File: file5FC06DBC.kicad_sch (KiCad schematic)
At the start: 29 parts, among them J7 SMA, U3 Si4463, U4 AS179-92LF, X1 TCXO 26 MHz

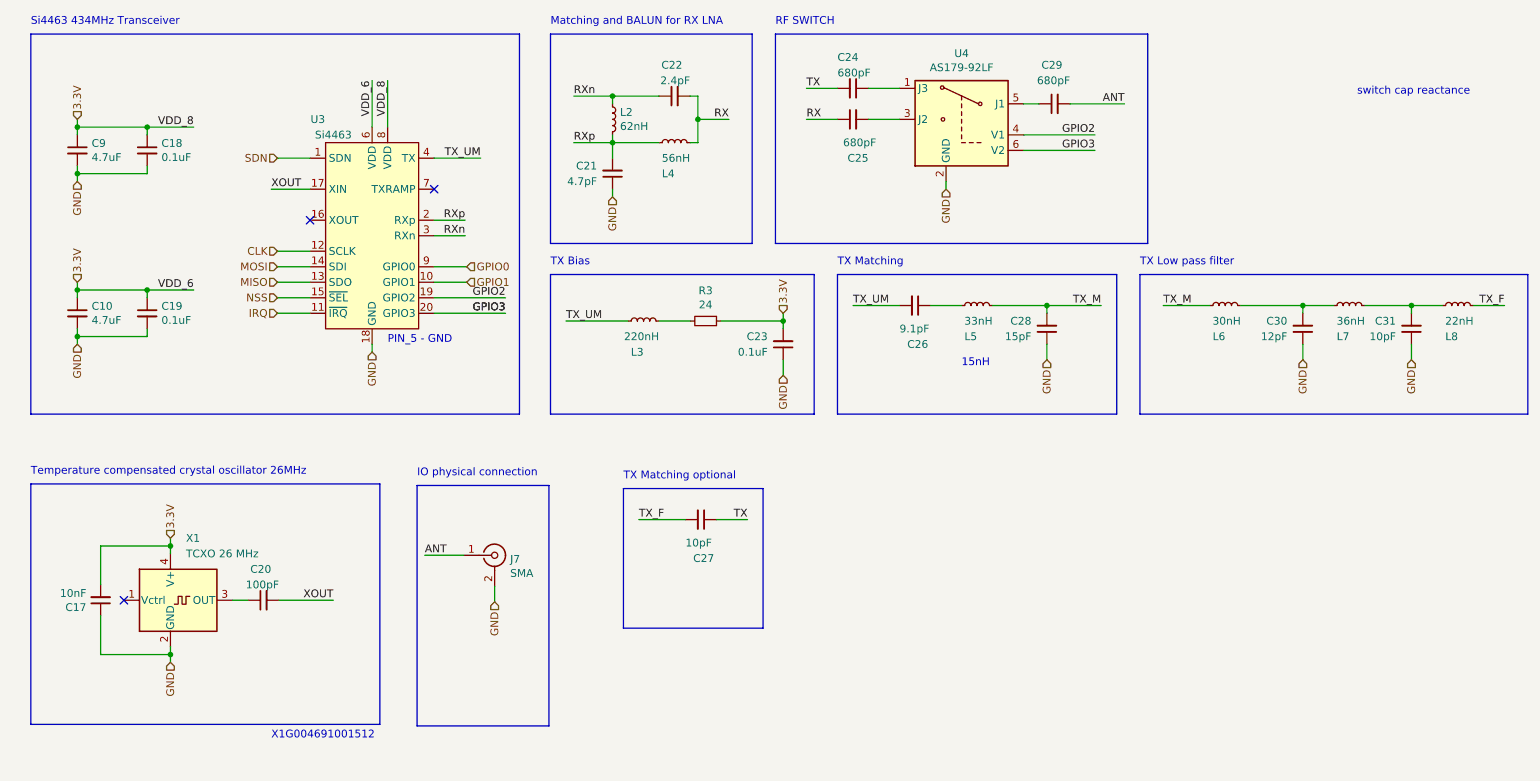
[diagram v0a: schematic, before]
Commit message: KiCad 0.2v
Schematics done.
Have to assign footprints to corresponding components.
Completely rework PCB.
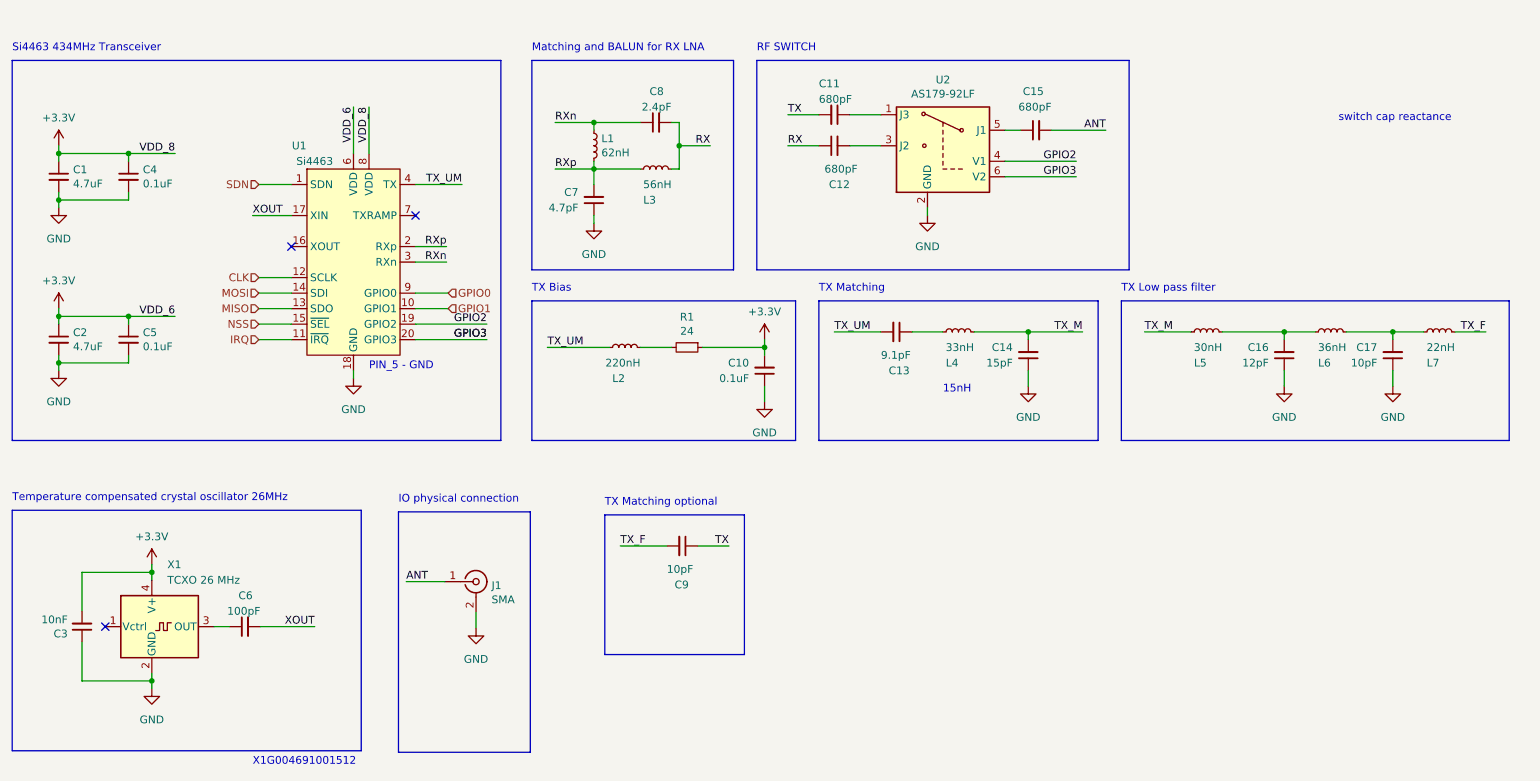
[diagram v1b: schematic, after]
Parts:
- removed C18, C19, C23: 0.1uF, Capacitor_SMD:C_0402_1005Metric, symbol Device:C_Small
- removed C20: 100pF, Capacitor_SMD:C_0402_1005Metric, symbol Device:C_Small
- removed C21: 4.7pF, Capacitor_SMD:C_0402_1005Metric, symbol Device:C_Small
- removed C22: 2.4pF, Capacitor_SMD:C_0402_1005Metric, symbol Device:C_Small
- removed C24, C25, C29: 680pF, Capacitor_SMD:C_0402_1005Metric, symbol Device:C_Small
- removed C26: 9.1pF, Capacitor_SMD:C_0402_1005Metric, symbol Device:C_Small
- removed C27, C31: 10pF, Capacitor_SMD:C_0402_1005Metric, symbol Device:C_Small
- removed C28: 15pF, Capacitor_SMD:C_0402_1005Metric, symbol Device:C_Small
- removed C30: 12pF, Capacitor_SMD:C_0402_1005Metric, symbol Device:C_Small
- removed J7: SMA, Connector_Coaxial:SMA_Molex_73251-1153_EdgeMount_Horizontal, symbol Connector:Conn_Coaxial
- removed L8: 22nH, Inductor_SMD:L_0402_1005Metric, symbol Device:L_Small
- removed R3: 24, Resistor_SMD:R_0603_1608Metric, symbol Device:R_Small
- removed U3: Si4463, Package_DFN_QFN:QFN-20-1EP_4x4mm_P0.5mm_EP2.6x2.6mm_ThermalVias, symbol RF:Si4463
- removed U4: AS179-92LF, Package_TO_SOT_SMD:SOT-363_SC-70-6, symbol RF_Switch:AS179-92LF
- added C1, C2: 4.7uF, Capacitor_SMD:C_0603_1608Metric, symbol Device:C_Small
- added C11, C12, C15: 680pF, Capacitor_SMD:C_0402_1005Metric, symbol Device:C_Small
- added C13: 9.1pF, Capacitor_SMD:C_0402_1005Metric, symbol Device:C_Small
- added C14: 15pF, Capacitor_SMD:C_0402_1005Metric, symbol Device:C_Small
- added C16: 12pF, Capacitor_SMD:C_0402_1005Metric, symbol Device:C_Small
- added C3: 10nF, Capacitor_SMD:C_0402_1005Metric, symbol Device:C_Small
- added C4, C5: 0.1uF, Capacitor_SMD:C_0402_1005Metric, symbol Device:C_Small
- added C6: 100pF, Capacitor_SMD:C_0402_1005Metric, symbol Device:C_Small
- added C7: 4.7pF, Capacitor_SMD:C_0402_1005Metric, symbol Device:C_Small
- added C8: 2.4pF, Capacitor_SMD:C_0402_1005Metric, symbol Device:C_Small
- added J1: SMA, Connector_Coaxial:SMA_Molex_73251-1153_EdgeMount_Horizontal, symbol Connector:Conn_Coaxial
- added L1: 62nH, Inductor_SMD:L_0402_1005Metric, symbol Device:L_Small
- added R1: 24, Resistor_SMD:R_0603_1608Metric, symbol Device:R_Small
- added U1: Si4463, Package_DFN_QFN:QFN-20-1EP_4x4mm_P0.5mm_EP2.6x2.6mm_ThermalVias, symbol RF:Si4463
- added U2: AS179-92LF, Package_TO_SOT_SMD:SOT-363_SC-70-6, symbol RF_Switch:AS179-92LF
- C10: value 4.7uF -> 0.1uF; footprint Capacitor_SMD:C_0603_1608Metric -> Capacitor_SMD:C_0402_1005Metric
- C17: value 10nF -> 10pF
- C9: value 4.7uF -> 10pF; footprint Capacitor_SMD:C_0603_1608Metric -> Capacitor_SMD:C_0402_1005Metric
- L2: value 62nH -> 220nH; footprint Inductor_SMD:L_0402_1005Metric -> Inductor_SMD:L_0603_1608Metric
- L3: value 220nH -> 56nH; footprint Inductor_SMD:L_0603_1608Metric -> Inductor_SMD:L_0402_1005Metric
- L4: value 56nH -> 33nH
- L5: value 33nH -> 30nH
- L6: value 30nH -> 36nH
- L7: value 36nH -> 22nH
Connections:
- net ANT: now also C15.2, J1.1 (In)
- net CLK: now also U1.12 (SCLK)
- net GND: now also C10.1, C1.2, C14.1, C16.1, C2.2, C3.1, C4.2, C5.2, C7.1, J1.2 (Ext), U1.18 (GND), U1.21 (GND), U2.2 (GND); no longer C10.2, C9.2
- net GPIO0: now also U1.9 (GPIO0)
- net GPIO1: now also U1.10 (GPIO1)
- net GPIO2: now also U1.19 (GPIO2), U2.4 (V1)
- net GPIO3: now also U1.20 (GPIO3), U2.6 (V2)
- net IRQ: now also U1.11 (~{IRQ})
- net MISO: now also U1.13 (SDO)
- net MOSI: now also U1.14 (SDI)
- net NSS: now also U1.15 (~{SEL})
- net RX: now also L3.2, C12.1, C8.2; no longer L4.2
- net RXn: now also C8.1, L1.1, U1.3 (RXn); no longer L2.1
- net RXp: now also L3.1, C7.2, L1.2, U1.2 (RXp); no longer L2.2, L4.1
- net SDN: now also U1.1 (SDN)
- net TX: now also C9.1, C11.2
- net TX_F: now also C9.2, L7.2
- net TX_M: now also L4.2, L5.1, C14.2; no longer L5.2, L6.1
- net TX_UM: now also L2.1, C13.2, U1.4 (TX); no longer L3.1
- net XOUT: now also C6.2, U1.17 (XIN)
- net at L6.2, L7.1: now also C17.2
- net at X1.3 (OUT): now also C6.1
- removed net 3.3V: C10.1, C17.2, C9.1, X1.4 (V+)
- new net: C12.2, U2.3 (J2)
- new net: C16.2, L5.2, L6.1
- new net: L2.2, R1.2
- new net: C11.1, U2.1 (J3)
- new net: C15.1, U2.5 (J1)
- new net: C13.1, L4.1
- new net +3V3: C1.1, C10.2, C2.1, C3.2, C4.1, C5.1, R1.1, U1.6 (VDD), U1.8 (VDD), X1.4 (V+)
